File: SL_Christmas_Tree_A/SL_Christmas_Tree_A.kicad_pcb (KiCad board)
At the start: 2 copper layers, 85.7 x 133.1 mm, 60 parts, among them J101 GND, J102 5V, J201 GND, J202 5V

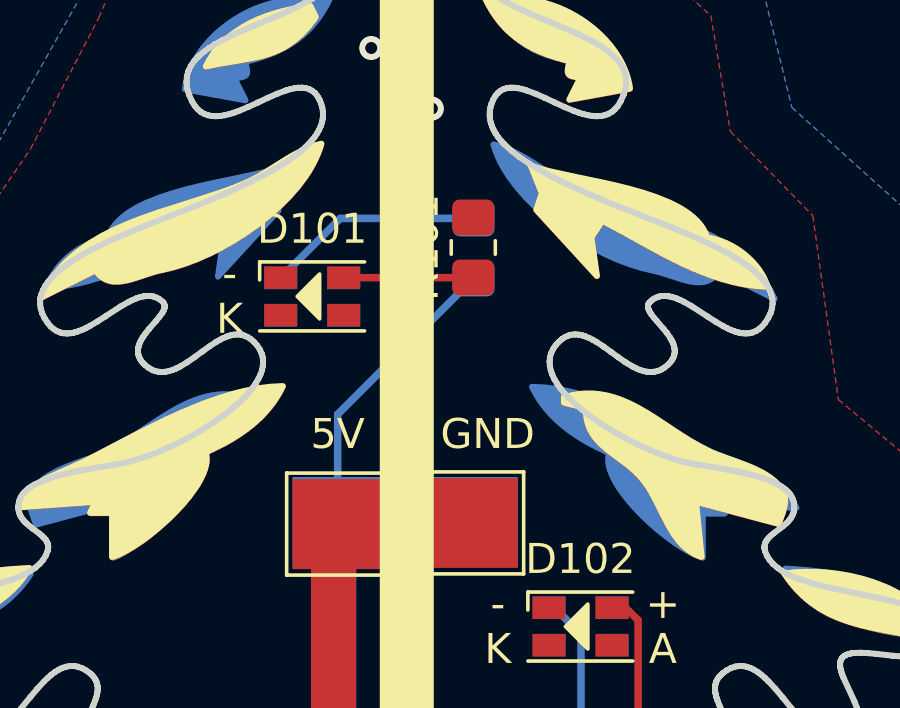
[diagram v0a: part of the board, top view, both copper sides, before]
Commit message: fixes
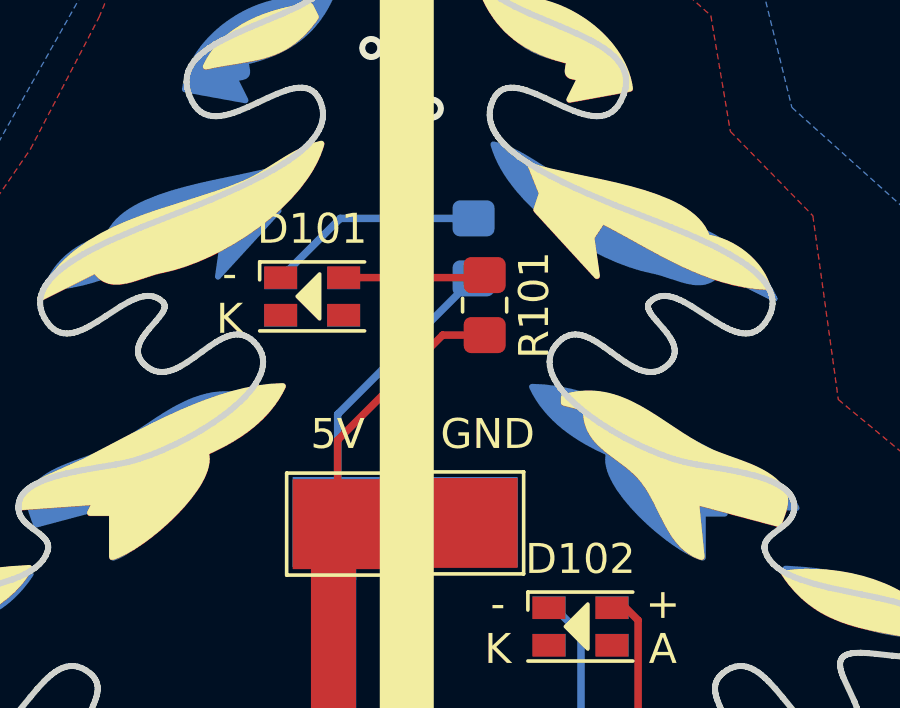
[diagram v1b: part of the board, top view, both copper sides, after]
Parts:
- moved R101 1.96 mm to (102.4, 68.2), turned to -90 degrees
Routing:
- net +5V: track 503.8 -> 513.0 mm
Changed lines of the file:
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@@
   )
   (footprint "Resistor_SMD:R_0805_2012Metric_Pad1.20x1.40mm_HandSolder" (layer "F.Cu")
-    (at 102.02 66.28 90)
+    (at 102.4 68.2 -90)
     (descr "Resistor SMD 0805 (2012 Metric), square (rectangular) end terminal, IPC_7351 nominal with elongated pad for handsoldering. (Body size source: IPC-SM-782 page 72, https://www.pcb-3d.com/wordpress/wp-content/uploads/ipc-sm-782a_amendment_1_and_2.pdf), generated with kicad-footprint-generator")
     (tags "resistor handsolder")
@@
     (fp_line (start 1 -0.625) (end 1 0.625) (layer "F.Fab") (width 0.1))
     (fp_line (start -1 -0.625) (end 1 -0.625) (layer "F.Fab") (width 0.1))
-    (pad "1" smd roundrect (at -1 0 90) (size 1.2 1.4) (layers "F.Cu" "F.Paste" "F.Mask") (roundrect_rratio 0.2083333333)
+    (pad "1" smd roundrect (at -1 0 270) (size 1.2 1.4) (layers "F.Cu" "F.Paste" "F.Mask") (roundrect_rratio 0.2083333333)
       (net 2 "Net-(D101-Pad2)") (pintype "passive"))
-    (pad "2" smd roundrect (at 1 0 90) (size 1.2 1.4) (layers "F.Cu" "F.Paste" "F.Mask") (roundrect_rratio 0.2083333333)
+    (pad "2" smd roundrect (at 1 0 270) (size 1.2 1.4) (layers "F.Cu" "F.Paste" "F.Mask") (roundrect_rratio 0.2083333333)
       (net 1 "+5V") (pintype "passive"))
     (model "${KICAD6_3DMODEL_DIR}/Resistor_SMD.3dshapes/R_0805_2012Metric.wrl"
@@
   (segment (start 97.36 85.61) (end 97.36 76.19) (width 1.5) (layer "F.Cu") (net 1))
   (segment (start 102.06 108.59) (end 102.06 109.81) (width 1.5) (layer "F.Cu") (net 1))
+  (segment (start 102.4 69.2) (end 101 69.2) (width 0.25) (layer "F.Cu") (net 1))
   (segment (start 97.37 163.29) (end 96.94 163.72) (width 1.5) (layer "F.Cu") (net 1))
   (segment (start 89.96 111.97) (end 97.33 111.97) (width 0.25) (layer "F.Cu") (net 1))
@@
   (segment (start 96.6 74.335717) (end 96.64952 74.286197) (width 0.25) (layer "F.Cu") (net 1))
   (segment (start 97.6 85.85) (end 97.36 85.61) (width 0.25) (layer "F.Cu") (net 1))
+  (segment (start 101 69.2) (end 97.5 72.7) (width 0.25) (layer "F.Cu") (net 1))
   (segment (start 107.92 109.18) (end 102.69 109.18) (width 0.25) (layer "F.Cu") (net 1))
   (segment (start 93.92 123.59) (end 86.6 130.91) (width 1.5) (layer "F.Cu") (net 1))
@@
   (segment (start 97.36 123.59) (end 93.92 123.59) (width 1.5) (layer "F.Cu") (net 1))
   (segment (start 116.68 135.26) (end 112.54 131.12) (width 0.25) (layer "F.Cu") (net 1))
+  (segment (start 97.5 72.7) (end 97.5 75.5) (width 0.25) (layer "F.Cu") (net 1))
   (via (at 97.37 119) (size 0.8) (drill 0.4) (layers "F.Cu" "B.Cu") (net 1))
   (via (at 102.06 108.59) (size 0.8) (drill 0.4) (layers "F.Cu" "B.Cu") (net 1))
